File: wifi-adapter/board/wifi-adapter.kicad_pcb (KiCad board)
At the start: 2 copper layers, 25 x 25 mm, 17 parts, among them J1 DF13A-6P-1.25H, U1 LM1117IMPX-3.3, U2 ESP-07

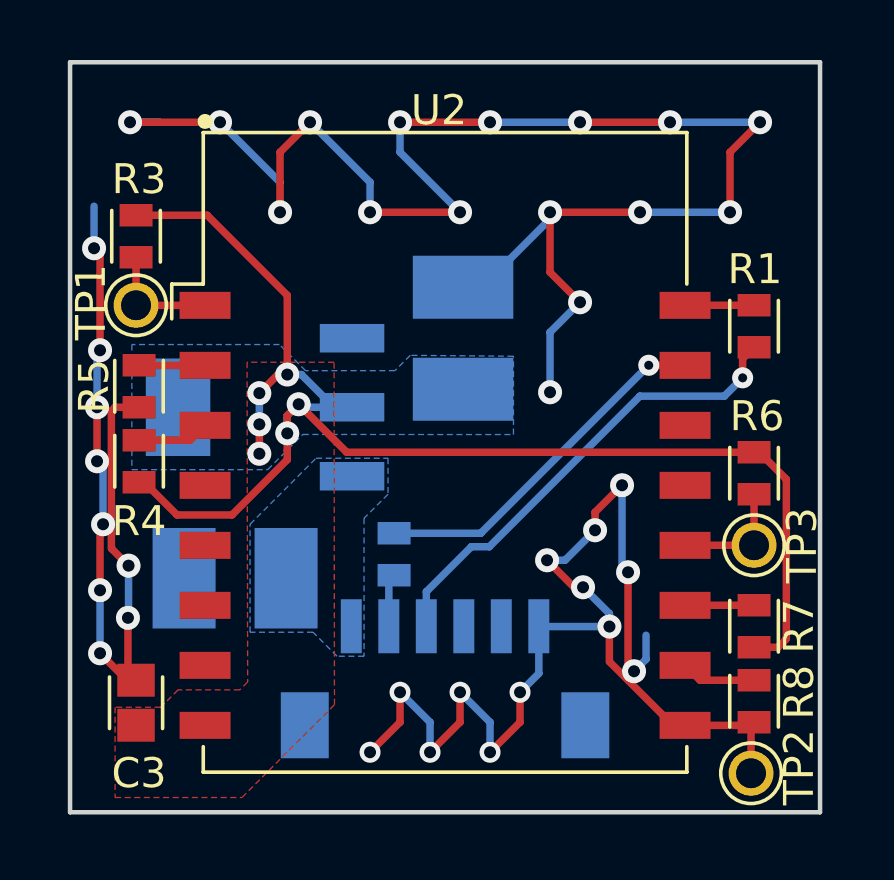
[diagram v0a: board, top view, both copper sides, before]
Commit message: Update to actual version
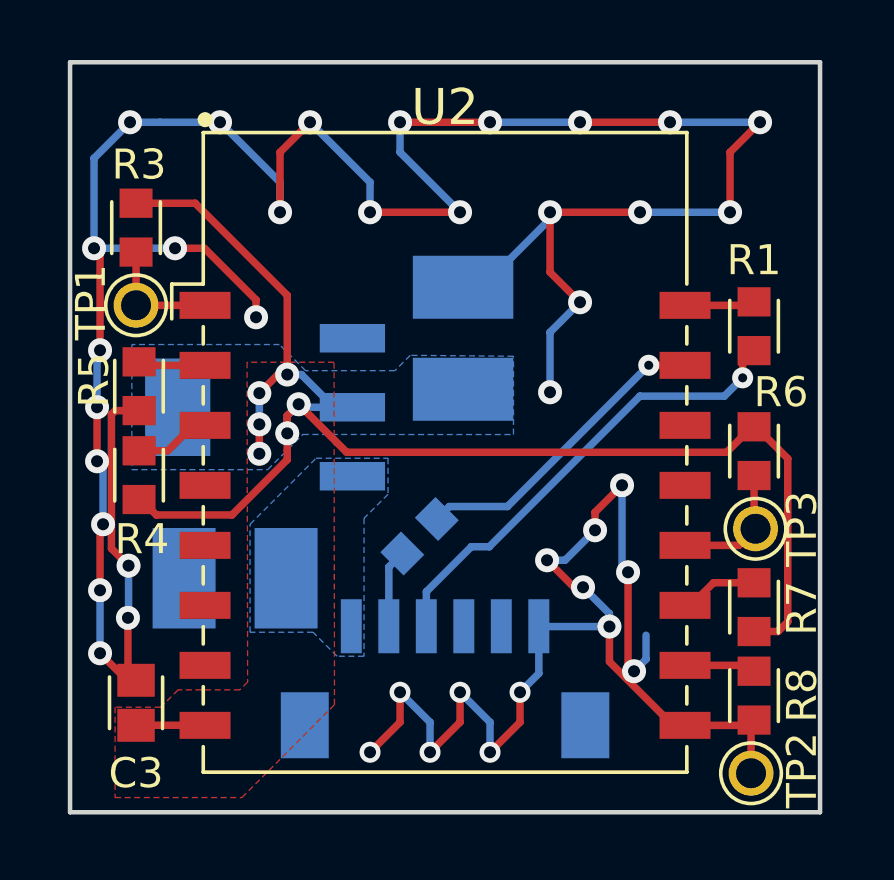
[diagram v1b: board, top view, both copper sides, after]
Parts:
- C1, C2: footprint spectrum:CAPC3225X230M -> wa:CAPC3225X230M
- C3: footprint spectrum:CAPC1608X92M -> wa:CAPC1608X92M
- J1: footprint spectrum:DF13A-6P-1.25H -> wa:HIROSE_DF13A-6P-1.25H
- R1, R2, R3, R4, R5, R6, R7, R8: footprint spectrum:RESC1608X55M -> wa:RESC1608X55M
- TP1, TP2, TP3: footprint spectrum:TP-TH-1 -> wa:TP-TH-1
- U1: footprint spectrum:SOT230P700X180-4M -> wa:SOT230P700X180-4M
- U2: footprint spectrum:SON200P2120X1600X300-16M -> wa:SON200P2120X1600X300-16M
- moved R2 1.04 mm to (147.7, 107.8), turned to 315 degrees
- moved R6 0.74 mm to (158.8, 105.0)
- moved R7 0.64 mm to (158.8, 110.2)
- moved TP3 0.55 mm to (158.8, 107.5)
- moved R4 0.46 mm to (138.3, 105.8)
- moved R3 0.29 mm to (138.2, 97.5)
- moved R8 0.19 mm to (158.8, 113.1)
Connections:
- J1 pad 4: Net-(J1-Pad4) -> (no net)
- J1 pad 5: Net-(J1-Pad5) -> (no net)
- J1 pad 7: Net-(J1-Pad7) -> (no net)
- J1 pad 8: Net-(J1-Pad8) -> (no net)
- U2 pad 13: Net-(U2-Pad13) -> (no net)
- U2 pad 14: Net-(U2-Pad14) -> (no net)
- U2 pad 4: Net-(U2-Pad4) -> (no net)
- U2 pad 5: Net-(U2-Pad5) -> (no net)
- U2 pad 6: Net-(U2-Pad6) -> (no net)
- U2 pad 7: Net-(U2-Pad7) -> (no net)
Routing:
- net GND: track 122.3 -> 131.5 mm, vias 38 -> 40
- net +3V3: track 49.5 -> 52.4 mm
- net Net-(R2-Pad2): track 12.0 -> 10.4 mm
- net /TELEM_TX: track 1.77 -> 2.61 mm
